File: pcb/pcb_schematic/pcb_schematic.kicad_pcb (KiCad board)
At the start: 4 copper layers, 41.5 x 48.4 mm, 35 parts, among them J1 Conn_ST_STDC14, J3 Conn_02x02_Odd_Even, J4 USB_B_Micro, Q1 MMBT3904, Q2 MMBT3904, Q3 MMBT3904, U1 STM32G031K8Tx, U2 NCP1117-3.3_SOT223, U4 SSD1306 128 x 64 OLED (0x3C), U5 TCS34725 (0x29), Y1 Crystal

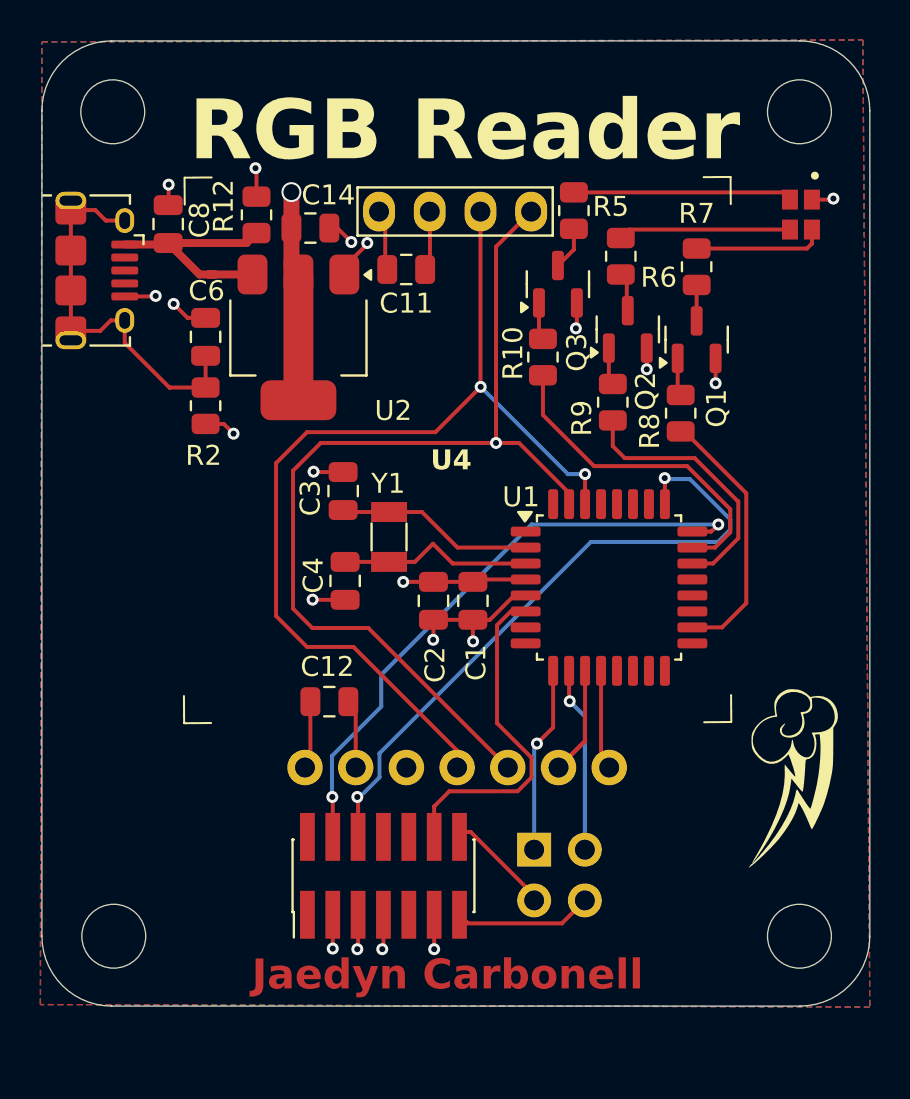
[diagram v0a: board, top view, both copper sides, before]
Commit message: ready to order :D
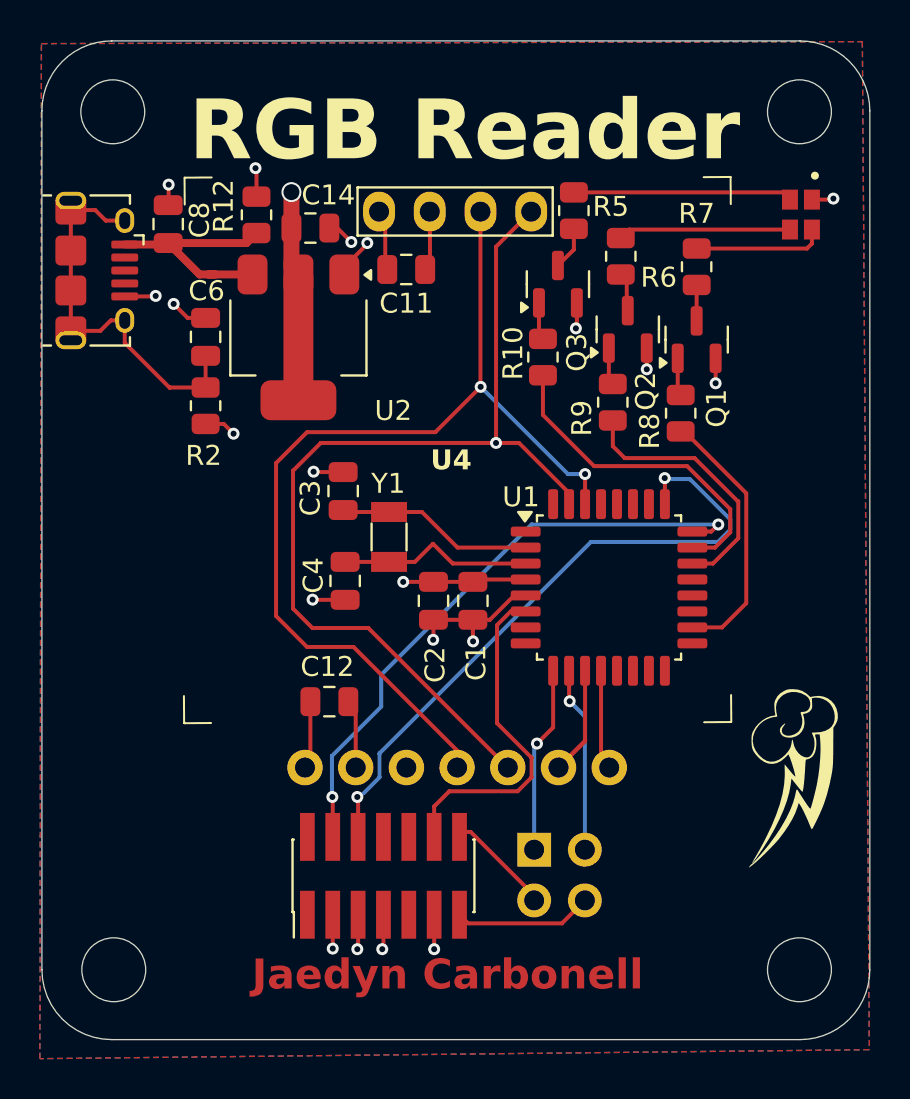
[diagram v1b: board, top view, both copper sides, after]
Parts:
- moved H3 1.68 mm to (136.9, 126.0)
- moved H4 1.68 mm to (171.2, 126.0)
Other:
- board size 41.5 x 48.4 mm -> 41.5 x 50 mm
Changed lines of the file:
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@@
 	(footprint "MountingHole:MountingHole_3.2mm_M3"
 		(layer "F.Cu")
-		(at 136.899293 124.314976)
+		(at 136.899293 125.994976)
 		(descr "Mounting Hole 3.2mm, no annular, M3")
 		(tags "mounting hole 3.2mm no annular m3")
@@
 	(footprint "MountingHole:MountingHole_3.2mm_M3"
 		(layer "F.Cu")
-		(at 171.249293 124.314976)
+		(at 171.249293 125.994976)
 		(descr "Mounting Hole 3.2mm, no annular, M3")
 		(tags "mounting hole 3.2mm no annular m3")
@@
 	)
 	(gr_line
-		(start 171.274293 127.814976)
-		(end 136.799293 127.814976)
-		(stroke
-			(width 0.05)
-			(type default)
-		)
-		(layer "Edge.Cuts")
-	)
-	(gr_line
-		(start 174.774293 82.964976)
-		(end 174.774293 124.314976)
+		(start 171.274293 129.494976)
+		(end 136.799293 129.494976)
 		(stroke
 			(width 0.05)
@@
 	)
 	(gr_arc
-		(start 136.799293 127.814976)
-		(mid 134.324419 126.78985)
-		(end 133.299293 124.314976)
+		(start 136.799293 129.494976)
+		(mid 134.324432 128.469846)
+		(end 133.299293 125.994976)
 		(stroke
 			(width 0.05)
@@
 	)
 	(gr_line
-		(start 136.799293 79.464976)
-		(end 171.274293 79.464976)
+		(start 133.299293 82.965)
+		(end 133.299293 125.994976)
 		(stroke
 			(width 0.05)
@@
 	)
 	(gr_line
-		(start 133.299293 124.314976)
-		(end 133.299293 82.964976)
+		(start 136.799293 79.464976)
+		(end 171.274293 79.464976)
 		(stroke
 			(width 0.05)
@@
 	)
 	(gr_arc
-		(start 174.774293 124.314976)
-		(mid 173.749167 126.78985)
-		(end 171.274293 127.814976)
+		(start 174.774293 125.994976)
+		(mid 173.749175 128.469863)
+		(end 171.274293 129.494976)
+		(stroke
+			(width 0.05)
+			(type default)
+		)
+		(layer "Edge.Cuts")
+	)
+	(gr_line
+		(start 174.774292 125.994976)
+		(end 174.774293 82.964976)
 		(stroke
 			(width 0.05)
@@
 		(polygon
 			(pts
-				(xy 133.299293 79.514976) (xy 174.424293 79.414976) (xy 174.774293 127.864976) (xy 133.224293 127.739976)
+				(xy 133.275 79.6) (xy 174.4 79.5) (xy 174.75 130) (xy 133.2 130.45)
 			)
 		)
@@
 		(polygon
 			(pts
-				(xy 133.843378 79.835526) (xy 133.843378 128.11837) (xy 175.268378 128.11837) (xy 175.268378 79.411098)
+				(xy 133.843378 79.835526) (xy 131.529751 130.431997) (xy 175.268378 130.3) (xy 175.268378 79.411098)
 			)
 		)
@@
 		(polygon
 			(pts
-				(xy 133.686828 79.719787) (xy 175.310215 79.706018) (xy 175.3 128.625) (xy 133.707251 128.583684)
+				(xy 133.686828 79.719787) (xy 175.310215 79.706018) (xy 175.3 130.275) (xy 131.858938 130.431997)
 			)
 		)
